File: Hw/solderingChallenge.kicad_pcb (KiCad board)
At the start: 2 copper layers, 13 parts, among them U1 ATtiny85-20SU

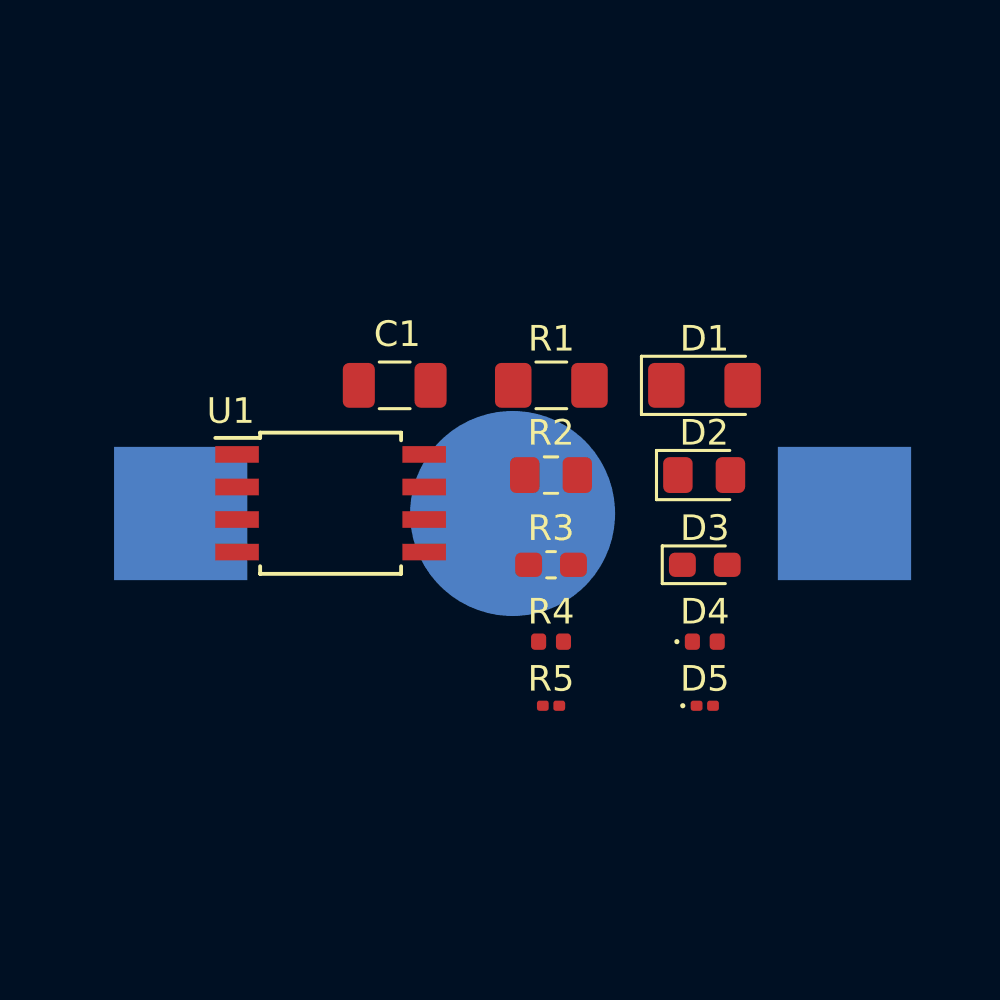
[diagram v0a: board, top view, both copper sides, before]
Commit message: Update connections
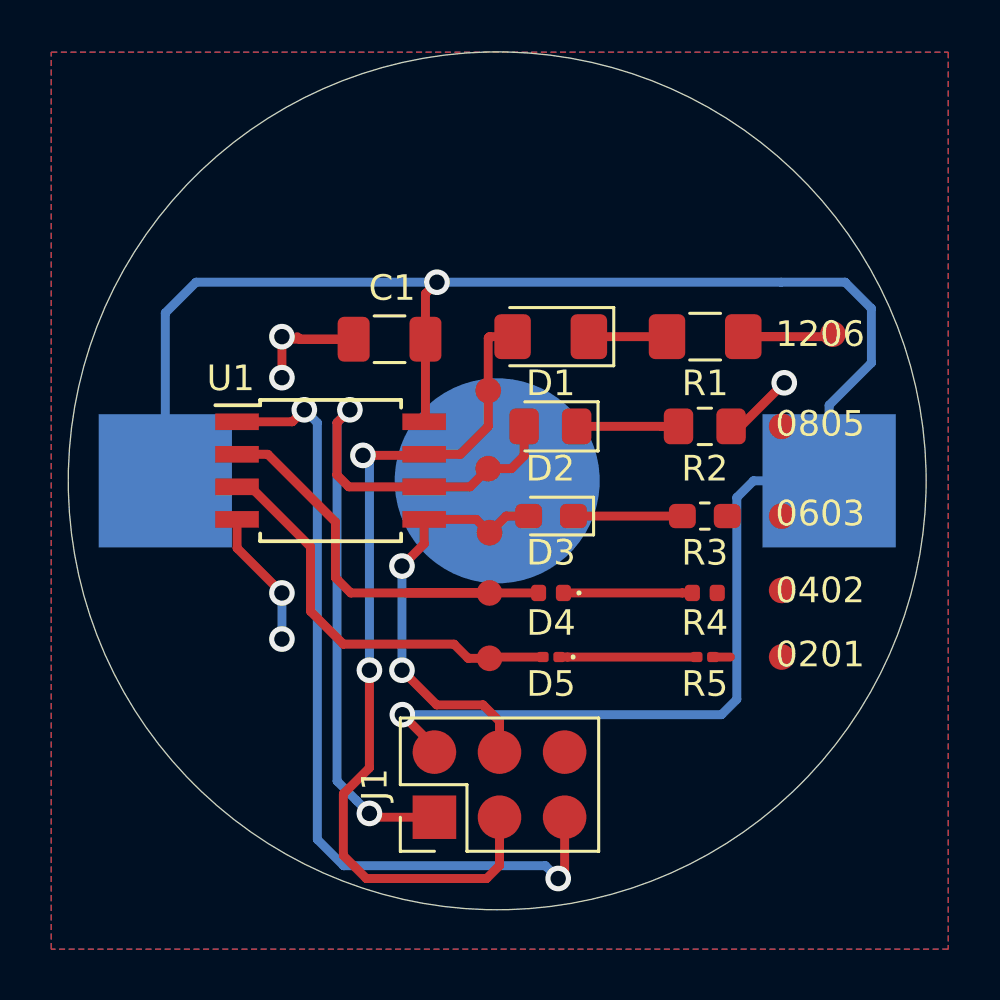
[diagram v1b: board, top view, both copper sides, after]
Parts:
- added J1: ISP, Connector_PinHeader_2.54mm:PinHeader_2x03_P2.54mm_Vertical, F.Cu at (139.9, 92.3)
- added TP1: PB0, TestPoint:TestPoint_Pad_1.0x1.0mm, F.Cu at (142.1, 81.2)
- added TP10: GND, Connectors_EC:TestPoint_Pad_1.0x1.0mm, F.Cu at (155.5, 73.5)
- added TP2: PB1, Connectors_EC:TestPoint_Pad_1.0x1.0mm, F.Cu at (142.1, 78.8)
- added TP3: PB2, Connectors_EC:TestPoint_Pad_1.0x1.0mm, F.Cu at (142.1, 75.7)
- added TP4: PB3, Connectors_EC:TestPoint_Pad_1.0x1.0mm, F.Cu at (142.1, 83.6)
- added TP5: PB4, Connectors_EC:TestPoint_Pad_1.0x1.0mm, F.Cu at (142.1, 86.2)
- added TP6: GND, Connectors_EC:TestPoint_Pad_1.0x1.0mm, F.Cu at (153.5, 83.5)
- added TP7: GND, Connectors_EC:TestPoint_Pad_1.0x1.0mm, F.Cu at (153.5, 77.1)
- added TP8: GND, Connectors_EC:TestPoint_Pad_1.0x1.0mm, F.Cu at (153.5, 80.6)
- added TP9: GND, Connectors_EC:TestPoint_Pad_1.0x1.0mm, F.Cu at (153.5, 86.1)
- moved D1 6.29 mm to (144.5, 73.6), turned to 180 degrees
- moved D2 6.29 mm to (144.5, 77.1), turned to 180 degrees
- moved D3 6.29 mm to (144.5, 80.6), turned to 180 degrees
- moved D4 6.29 mm to (144.5, 83.6), turned to 180 degrees
- moved D5 6.29 mm to (144.5, 86.1), turned to 180 degrees
- moved R1 6.29 mm to (150.5, 73.6), turned to 180 degrees
- moved R2 6.29 mm to (150.5, 77.1), turned to 180 degrees
- moved R3 6.29 mm to (150.5, 80.6), turned to 180 degrees
- moved R4 6.29 mm to (150.5, 83.6), turned to 180 degrees
- moved R5 6.29 mm to (150.5, 86.1), turned to 180 degrees
- moved C1 1.81 mm to (138.2, 73.7)
- moved BT1 1.41 mm to (142.4, 79.2)
- moved U1 1.27 mm to (135.9, 78.8)
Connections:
- net /PB1 renamed /MISO
- D1 pad 2: /PB0 -> /PB2
- D3 pad 2: /PB2 -> /MOSI
- U1 pad 5: /PB0 -> /MOSI
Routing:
- net VCC: track 0.00 -> 75.1 mm, vias 0 -> 2
- net /PB2: track 0.00 -> 34.5 mm, vias 0 -> 2
- net /RST: track 0.00 -> 32.3 mm, vias 0 -> 2
- net /MISO: track 0.00 -> 31.0 mm, vias 0 -> 2
- net GND: track 0.00 -> 20.7 mm, vias 0 -> 5
- net /PB3: track 0.00 -> 18.5 mm
- net /MOSI: track 0.00 -> 16.8 mm, vias 0 -> 2
- net /PB4: track 0.00 -> 16.2 mm
- net Net-(D5-Pad1): track 0.00 -> 5.36 mm
- net Net-(D4-Pad1): track 0.00 -> 5.03 mm
- net Net-(D3-Pad1): track 0.00 -> 4.25 mm
- net Net-(D2-Pad1): track 0.00 -> 3.97 mm
- net Net-(D1-Pad1): track 0.00 -> 3.05 mm
- added copper zone on B.Cu, net GND
- added copper zone on F.Cu, net GND
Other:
- board outline added: 33.5 x 33.5 mm
- net class Default: trace_width 0.25 -> 0.35; via_dia 0.8 -> 1; via_drill 0.4 -> 0.6
- net class vcc added: clearance 0.3, trace_width 0.5, via_dia 1, via_drill 0.6
- rule trace_min: 0.2 -> 0.3
- board text added: "0201"
- board text added: "0402"
- board text added: "0603"
- board text added: "0805"
- board text added: "1206"
